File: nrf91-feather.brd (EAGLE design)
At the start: 50.8 x 22.9 mm, 123 parts, among them J2 CON-HEADER-1X12-MALE-PIN, J3 CON-HEADER-1X16-MALE-PIN, J4 CON-1909763-1, J5 CON-SIM-104224-0820, J6 CON-S2B-PH-SM4-TB(LF)(SN), J7 CON-1909763-1, J8 CON-USB-DX07S016JA1R1500, J9 CON-TC2030-MCP-NL, Q2 MOSFET-DUAL-COMP-SOT563, Q3 MOSFET-P-20V-4.7A-SOT23, Q4 MOSFET-N-SC89, Q5 MOSFET-N-SC89, SW1 SW-EVP-AA402W, SW2 SW-EVP-AA402W, U1 MOD-NRF9160-SICA-R, U10 IC-LIS2DH12TR, U2 IC-CP2102N-A02-GQFN20R, U3 IC-TPS62840DLCR, U4 POWER-SWITCH-MIC94092YC6, U5 IC-MCP73830T, U6 FLASH-W25Q32JVZPIQ-WSON, U8 IC-PCF85063ATL/1, Y1 XTAL-ABS07AIG-32.768KHZ-7-T

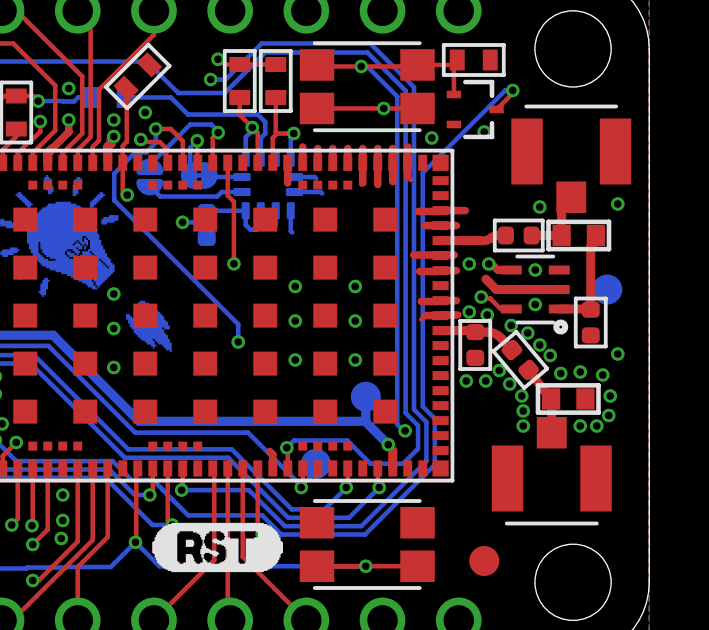
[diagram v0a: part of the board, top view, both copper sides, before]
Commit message: V5 Proto 1
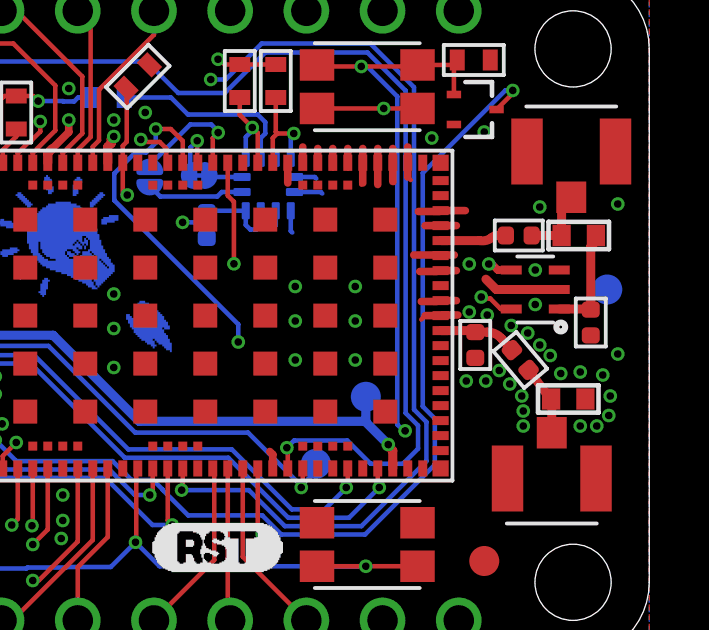
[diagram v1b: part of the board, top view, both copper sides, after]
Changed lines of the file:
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@@
 <layer number="49" name="Reference" color="7" fill="1" visible="no" active="yes"/>
 <layer number="50" name="dxf" color="7" fill="1" visible="no" active="no"/>
-<layer number="51" name="tDocu" color="7" fill="1" visible="yes" active="yes"/>
+<layer number="51" name="tDocu" color="7" fill="1" visible="no" active="yes"/>
 <layer number="52" name="bDocu" color="7" fill="1" visible="no" active="yes"/>
 <layer number="53" name="tGND_GNDA" color="7" fill="9" visible="no" active="no"/>
@@
 <wire x1="27.72" y1="14.43" x2="27.5" y2="14.21" width="0.254" layer="1"/>
 <wire x1="27.5" y1="14.21" x2="27.5" y2="13.95" width="0.254" layer="1"/>
-<wire x1="43.9" y1="11.45" x2="44.42" y2="11.45" width="0.254" layer="1"/>
-<wire x1="43.845" y1="11.43" x2="43.9" y2="11.45" width="0" layer="19" extent="1-1"/>
+<wire x1="43.9" y1="11.45" x2="44.05" y2="11.45" width="0.254" layer="1"/>
+<wire x1="44.05" y1="11.45" x2="44.42" y2="11.45" width="0.254" layer="1"/>
+<wire x1="43.845" y1="11.43" x2="43.865" y2="11.45" width="0.1524" layer="1"/>
+<wire x1="43.865" y1="11.45" x2="44.05" y2="11.45" width="0.1524" layer="1"/>
 </signal>
 <signal name="+3V3">
